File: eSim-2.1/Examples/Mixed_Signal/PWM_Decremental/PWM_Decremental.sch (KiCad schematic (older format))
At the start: 16 parts, among them U1 plot_v1, U2 pwmdecrement, U3 plot_v1, U4 adc_bridge_1, U5 adc_bridge_1, U6 plot_v1, U7 plot_v1, U8 dac_bridge_1, U9 plot_v1, X1 lm_741

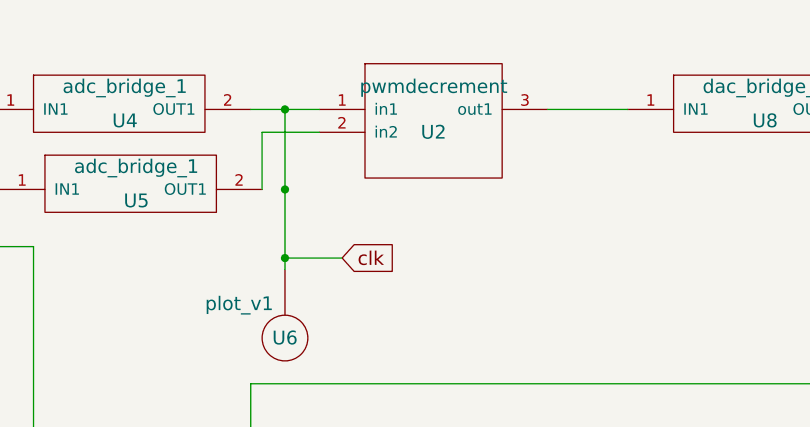
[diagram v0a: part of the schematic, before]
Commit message: Ngveri update
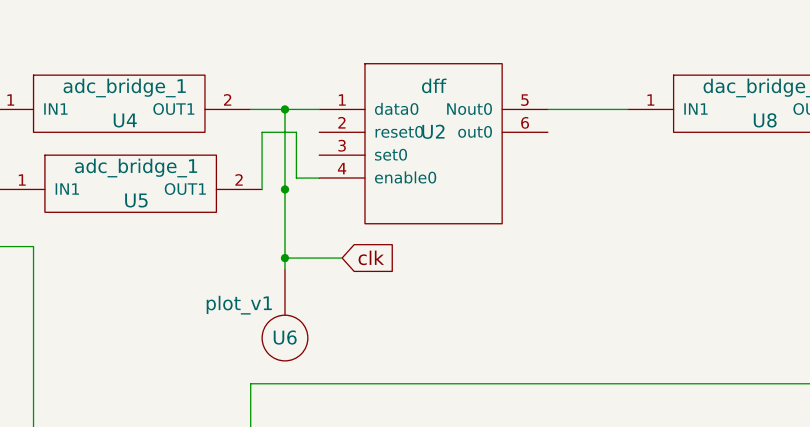
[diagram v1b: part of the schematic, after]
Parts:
- removed U2: pwmdecrement, symbol pwmdecrement
- added U2: dff, symbol dff
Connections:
- net clk: now also U2.1 (data0)
- net at U8.1 (IN1): now also U2.5 (Nout0)
- net at U5.2 (OUT1): now also U2.4 (enable0)
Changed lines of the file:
@@
 EESchema Schematic File Version 2
+LIBS:PWM_Decremental-rescue
 LIBS:power
 LIBS:switches
@@
 LIBS:eSim_Plot
 LIBS:eSim_Nghdl
+LIBS:eSim_Ngveri
 LIBS:PWM_Decremental-cache
 EELAYER 25 0
@@
 $EndComp
 $Comp
-L eSim_GND #PWR3
+L eSim_GND #PWR01
 U 1 1 5DCD9465
 P 3300 5150
-F 0 "#PWR3" H 3300 4900 50  0001 C CNN
+F 0 "#PWR01" H 3300 4900 50  0001 C CNN
 F 1 "eSim_GND" H 3300 5000 50  0000 C CNN
 F 2 "" H 3300 5150 50  0001 C CNN
@@
 $EndComp
 $Comp
-L eSim_GND #PWR2
+L eSim_GND #PWR02
 U 1 1 5DCD9466
 P 2700 3300
-F 0 "#PWR2" H 2700 3050 50  0001 C CNN
+F 0 "#PWR02" H 2700 3050 50  0001 C CNN
 F 1 "eSim_GND" H 2700 3150 50  0000 C CNN
 F 2 "" H 2700 3300 50  0001 C CNN
@@
 $EndComp
 $Comp
-L eSim_GND #PWR1
+L eSim_GND #PWR03
 U 1 1 5DCD9468
 P 1600 3900
-F 0 "#PWR1" H 1600 3650 50  0001 C CNN
+F 0 "#PWR03" H 1600 3650 50  0001 C CNN
 F 1 "eSim_GND" H 1600 3750 50  0000 C CNN
 F 2 "" H 1600 3900 50  0001 C CNN
@@
 $EndComp
 $Comp
-L eSim_GND #PWR4
+L eSim_GND #PWR04
 U 1 1 5DCD946D
 P 4500 3150
-F 0 "#PWR4" H 4500 2900 50  0001 C CNN
+F 0 "#PWR04" H 4500 2900 50  0001 C CNN
 F 1 "eSim_GND" H 4500 3000 50  0000 C CNN
 F 2 "" H 4500 3150 50  0001 C CNN
@@
 clk
 $Comp
-L eSim_GND #PWR5
+L eSim_GND #PWR05
 U 1 1 5DCD9470
 P 6850 5450
-F 0 "#PWR5" H 6850 5200 50  0001 C CNN
+F 0 "#PWR05" H 6850 5200 50  0001 C CNN
 F 1 "eSim_GND" H 6850 5300 50  0000 C CNN
 F 2 "" H 6850 5450 50  0001 C CNN
@@
 Connection ~ 6250 1850
 Wire Wire Line
-	6400 1950 6150 1950
-Wire Wire Line
 	6150 1950 6150 2200
 Wire Notes Line
@@
 Wire Wire Line
 	9300 6400 9300 4500
-$Comp
-L pwmdecrement U2
-U 1 1 61078941
+Wire Wire Line
+	6400 2150 6300 2150
+Wire Wire Line
+	6300 2150 6300 1950
+Wire Wire Line
+	6300 1950 6150 1950
+$Comp
+L dff U2
+U 1 1 6123E15B
 P 4050 3750
 F 0 "U2" H 6900 5550 60  0000 C CNN
-F 1 "pwmdecrement" H 6900 5750 60  0000 C CNN
+F 1 "dff" H 6900 5750 60  0000 C CNN
 F 2 "" H 6900 5700 60  0000 C CNN
 F 3 "" H 6900 5700 60  0000 C CNN
